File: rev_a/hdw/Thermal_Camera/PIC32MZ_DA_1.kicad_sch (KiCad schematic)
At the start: 3 parts, among them U1701 PIC32MZ2064DAR176

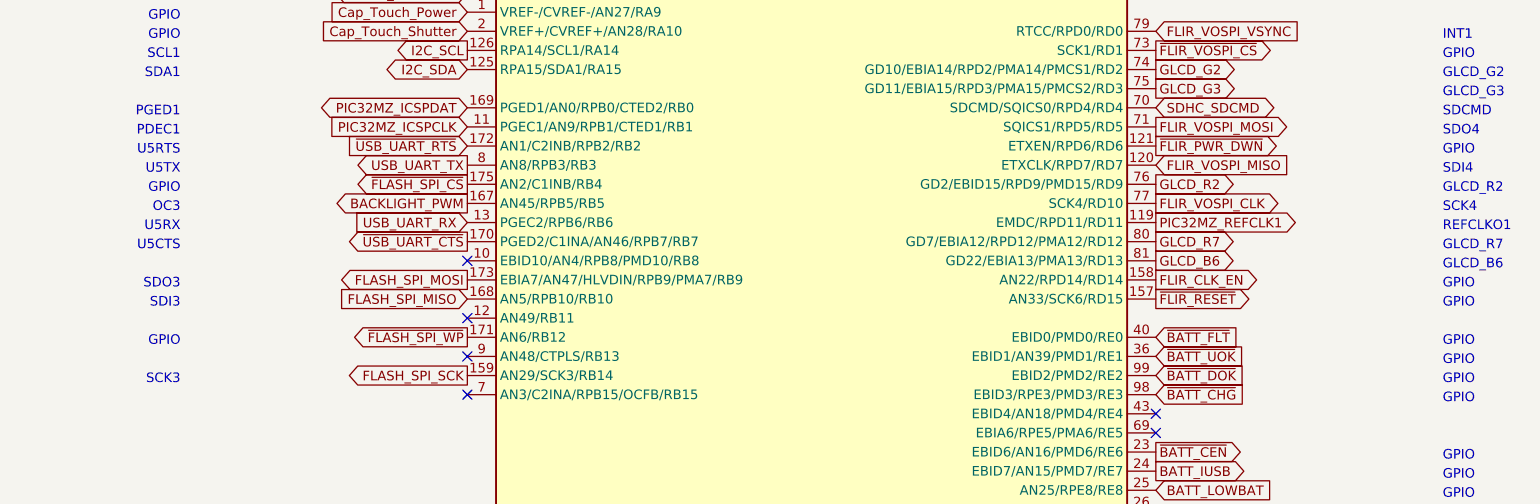
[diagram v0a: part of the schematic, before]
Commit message: some more routing, moved some misc nets on MCU
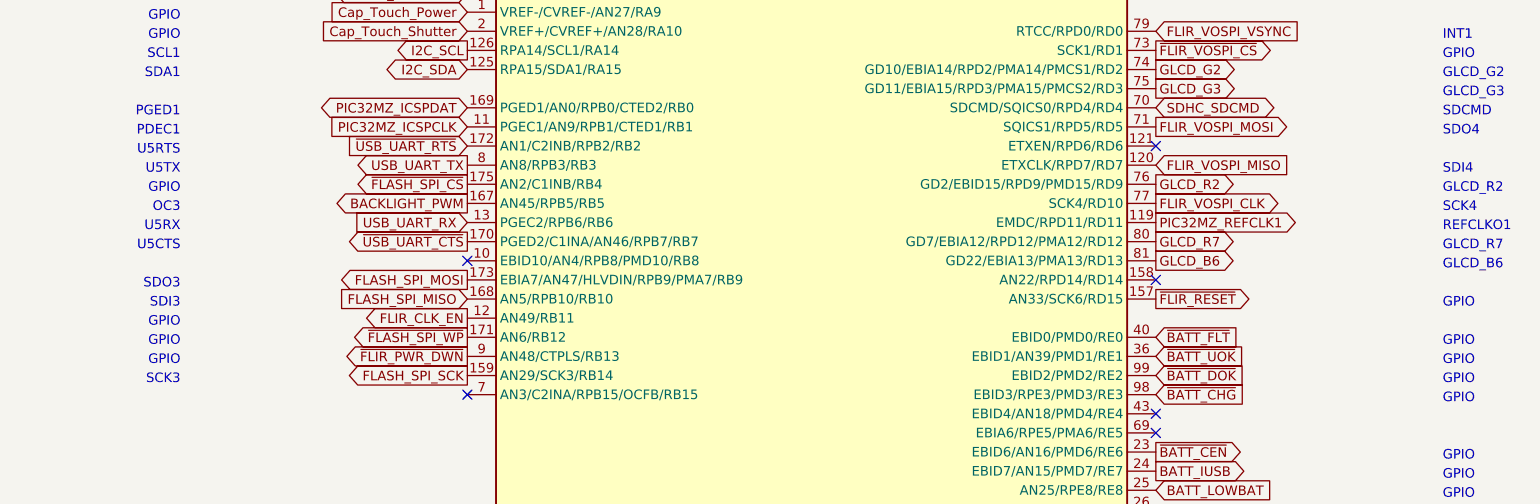
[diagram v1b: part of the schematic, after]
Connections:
- net FLIR_CLK_EN: now also U1701.12 (AN49/RB11); no longer U1701.158 (AN22/RPD14/RD14)
- net ~{FLIR_PWR_DWN}: now also U1701.9 (AN48/CTPLS/RB13); no longer U1701.121 (ETXEN/RPD6/RD6)
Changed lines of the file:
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@@
+	)
+	(no_connect
+		(at 182.88 82.55)
+	)
+	(no_connect
+		(at 91.44 57.15)
+	)
+	(no_connect
+		(at 182.88 130.81)
+	)
+	(no_connect
+		(at 182.88 57.15)
+	)
+	(no_connect
+		(at 91.44 52.07)
+	)
+	(no_connect
+		(at 182.88 100.33)
+	)
+	(no_connect
+		(at 182.88 120.65)
+	)
+	(no_connect
+		(at 91.44 46.99)
+	)
+	(no_connect
+		(at 91.44 97.79)
 	)
 	(no_connect
@@
 	)
 	(no_connect
-		(at 91.44 57.15)
-	)
-	(no_connect
-		(at 182.88 130.81)
-	)
-	(no_connect
-		(at 182.88 57.15)
-	)
-	(no_connect
-		(at 91.44 105.41)
-	)
-	(no_connect
-		(at 91.44 52.07)
-	)
-	(no_connect
-		(at 182.88 120.65)
-	)
-	(no_connect
-		(at 91.44 46.99)
-	)
-	(no_connect
-		(at 91.44 110.49)
-	)
-	(no_connect
-		(at 91.44 97.79)
-	)
-	(no_connect
 		(at 91.44 49.53)
 	)
@@
 		)
 	)
+	(text "GPIO"
+		(exclude_from_sim no)
+		(at 53.34 111.76 0)
+		(effects
+			(font
+				(size 1.27 1.27)
+			)
+			(justify right bottom)
+		)
+	)
 	(text "POSC"
 		(exclude_from_sim no)
@@
 		)
 	)
-	(text "GPIO"
-		(exclude_from_sim no)
-		(at 220.98 83.82 0)
-		(effects
-			(font
-				(size 1.27 1.27)
-			)
-			(justify left bottom)
-		)
-	)
 	(text "U5TX"
 		(exclude_from_sim no)
@@
 		)
 	)
-	(text "GPIO"
-		(exclude_from_sim no)
-		(at 220.98 101.6 0)
-		(effects
-			(font
-				(size 1.27 1.27)
-			)
-			(justify left bottom)
-		)
-	)
 	(text "OC3"
 		(exclude_from_sim no)
@@
 		(exclude_from_sim no)
 		(at 53.34 55.88 0)
+		(effects
+			(font
+				(size 1.27 1.27)
+			)
+			(justify right bottom)
+		)
+	)
+	(text "GPIO"
+		(exclude_from_sim no)
+		(at 53.34 106.68 0)
 		(effects
 			(font
@@
 	(global_label "~{FLIR_PWR_DWN}"
 		(shape output)
-		(at 182.88 82.55 0)
-		(fields_autoplaced yes)
-		(effects
-			(font
-				(size 1.27 1.27)
-			)
-			(justify left)
-		)
-		(property "Intersheetrefs" "${INTERSHEET_REFS}"
-			(at 199.8352 82.55 0)
-			(effects
-				(font
-					(size 1.27 1.27)
-				)
-				(justify left)
+		(at 91.44 110.49 180)
+		(fields_autoplaced yes)
+		(effects
+			(font
+				(size 1.27 1.27)
+			)
+			(justify right)
+		)
+		(property "Intersheetrefs" "${INTERSHEET_REFS}"
+			(at 74.4848 110.49 0)
+			(effects
+				(font
+					(size 1.27 1.27)
+				)
+				(justify right)
 				(hide yes)
 			)
@@
 	(global_label "FLIR_CLK_EN"
 		(shape output)
-		(at 182.88 100.33 0)
-		(fields_autoplaced yes)
-		(effects
-			(font
-				(size 1.27 1.27)
-			)
-			(justify left)
-		)
-		(property "Intersheetrefs" "${INTERSHEET_REFS}"
-			(at 197.8395 100.33 0)
-			(effects
-				(font
-					(size 1.27 1.27)
-				)
-				(justify left)
-				(hide yes)
-			)
+		(at 91.44 105.41 180)
+		(fields_autoplaced yes)
+		(effects
+			(font
+				(size 1.27 1.27)
+			)
+			(justify right)
+		)
+		(property "Intersheetrefs" "${INTERSHEET_REFS}"
+			(at 76.4805 105.41 0)
+			(effects
+				(font
+					(size 1.27 1.27)
+				)
+				(justify right)
+				(hide yes)
+			)
